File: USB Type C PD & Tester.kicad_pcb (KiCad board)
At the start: 2 copper layers, 115 x 50 mm, 61 parts, among them J1 USB_B_Micro, J3 USB_C_Receptacle_USB2.0_14P, J4 Screw_Terminal_01x02, Q1 BSD840N, Q2 BSD840N, Q3 BSD840N, Q4 BSD840N, SW1 SW_Push, U1 MIC5504-1.2YM5, U2 STM32F072CBTx, U3 INA237, U4 INA237, U5 AD8606ARM, U6 FUSB302B01MPX

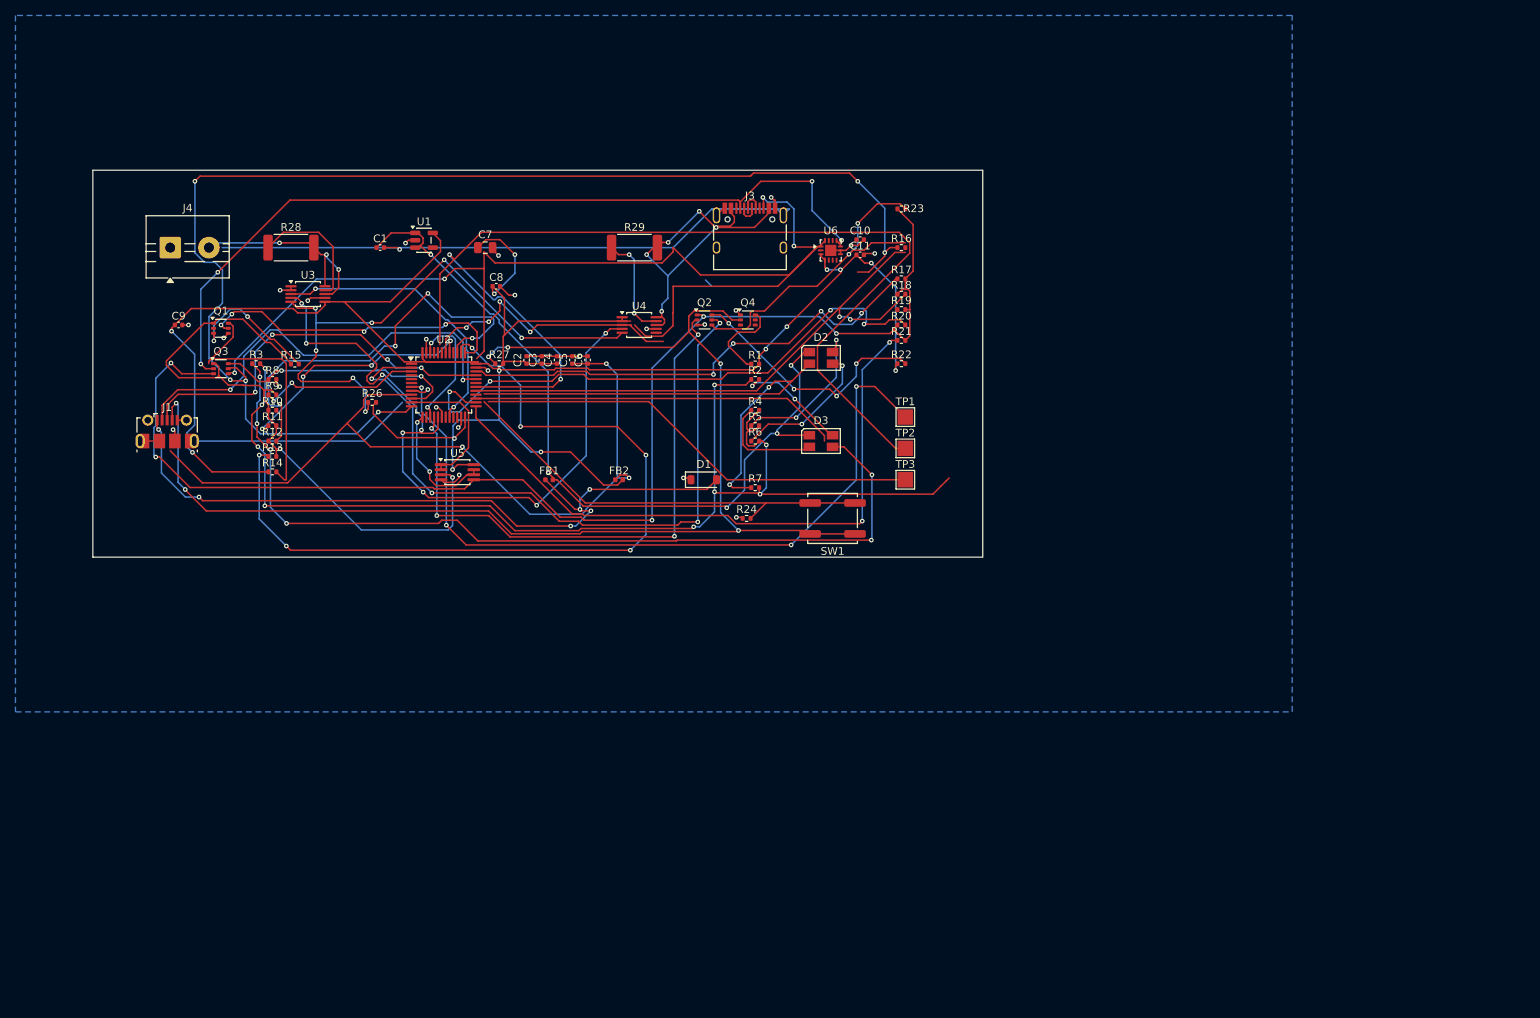
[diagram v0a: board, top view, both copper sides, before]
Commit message: Add files via upload
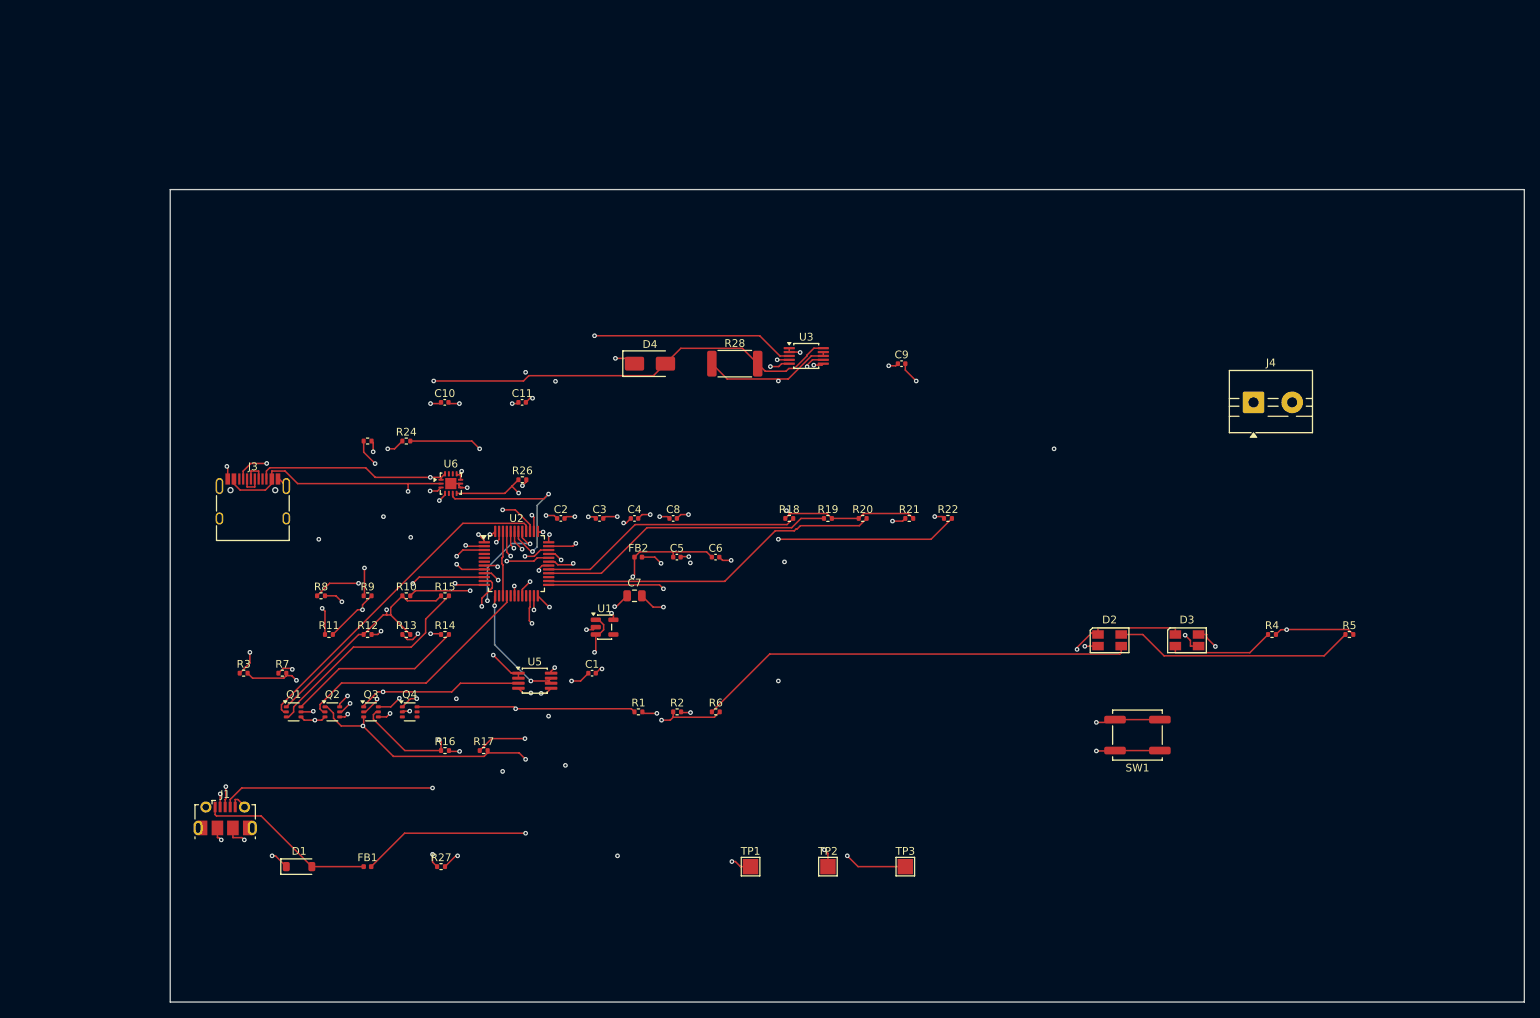
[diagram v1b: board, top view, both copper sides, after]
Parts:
- removed R29: 0.012Ω, Resistor_SMD:R_2512_6332Metric
- removed U4: INA237, Package_SO:VSSOP-10_3x3mm_P0.5mm
- added D4: D_TVS, Diode_SMD:D_SMA, F.Cu at (107.0, 65.0)
- moved J4 141.4 mm to (185.0, 70.0)
- moved C9 93.6 mm to (139.5, 65.0)
- moved R16 87.8 mm to (80.5, 115.0)
- moved R17 81.4 mm to (85.5, 115.0)
- moved R5 81.4 mm to (197.4, 100.0)
- moved R23 75.2 mm to (70.5, 75.0)
- moved J3 73.2 mm to (55.7, 84.0)
- moved R4 72.8 mm to (187.4, 100.0)
- moved D1 72.4 mm to (61.6, 130.0)
- moved Q2 69.9 mm to (66.0, 110.0)
- moved Q4 66.9 mm to (76.0, 110.0)
- moved R7 65.6 mm to (59.5, 105.0)
- moved R27 65.4 mm to (80.0, 130.0)
- moved U3 64.9 mm to (127.2, 64.0)
- moved TP1 61.4 mm to (120.0, 130.0)
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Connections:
- R26 pad 1: /INA_SDA -> INA_SDA
- R28 pad 1: Net-(U3-Vin-) -> /VBUS_PLUG
- R28 pad 2: /VBUS_PLUG -> /VBUS_RECEP
- U2 pad 17: /VCONN_ALERT_L -> unconnected-(U2-PA7-Pad17)
- U2 pad 42: /INA_SCL -> INA_SCL
- U2 pad 43: /INA_SDA -> INA_SDA
- U3 pad 10: /VBUS_PLUG -> /VBUS_RECEP
- U3 pad 4: /VCONN_ALERT_L -> INA_SDA
- U3 pad 5: /INA_SDA -> INA_SCL
- U3 pad 9: Net-(U3-Vin-) -> /VBUS_PLUG
- U6 pad 6: /INA_SCL -> INA_SCL
- U6 pad 7: /INA_SDA -> INA_SDA
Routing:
- net +3V3: track 287.6 -> 33.0 mm, vias 14 -> 23
- net /CC2_EN: track 167.9 -> 38.2 mm, vias 6 -> 2
- net GND: track 172.6 -> 70.9 mm, vias 25 -> 31
- net /VCONN_ALERT_L: track 91.3 -> 0.00 mm, vias 8 -> 0
- net /CC2_RECEP: track 149.3 -> 59.6 mm, vias 4 -> 2
- net /INA_SDA: track 74.8 -> 0.00 mm, vias 7 -> 0
- net Net-(R24-Pad2): track 56.2 -> 129.6 mm, vias 0 -> 3
- net /CC1_RPUSB: track 106.1 -> 34.5 mm, vias 6 -> 3
- net INA_SCL: track 0.00 -> 71.0 mm, vias 0 -> 4
- net INA_SDA: track 0.00 -> 70.9 mm, vias 0 -> 4
- net Net-(D1-A): track 93.8 -> 23.0 mm, vias 6 -> 0
- net Net-(U2-VDDA): track 103.0 -> 33.6 mm, vias 3 -> 2
- net /UART_TX: track 145.1 -> 75.7 mm, vias 2 -> 3
- net Net-(Q2A-D): track 32.6 -> 100.2 mm, vias 4 -> 3
- net Net-(D3-RK): track 14.6 -> 75.7 mm
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- added copper zone on In2.Cu, net +3V3
- added copper zone on In1.Cu, net GND
- removed copper zone on B.Cu, net GND
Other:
- board size 115 x 50 mm -> 175 x 105 mm
- copper layers 2 -> 4
- board text removed: "${REFERENCE}"

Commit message: Add files via upload
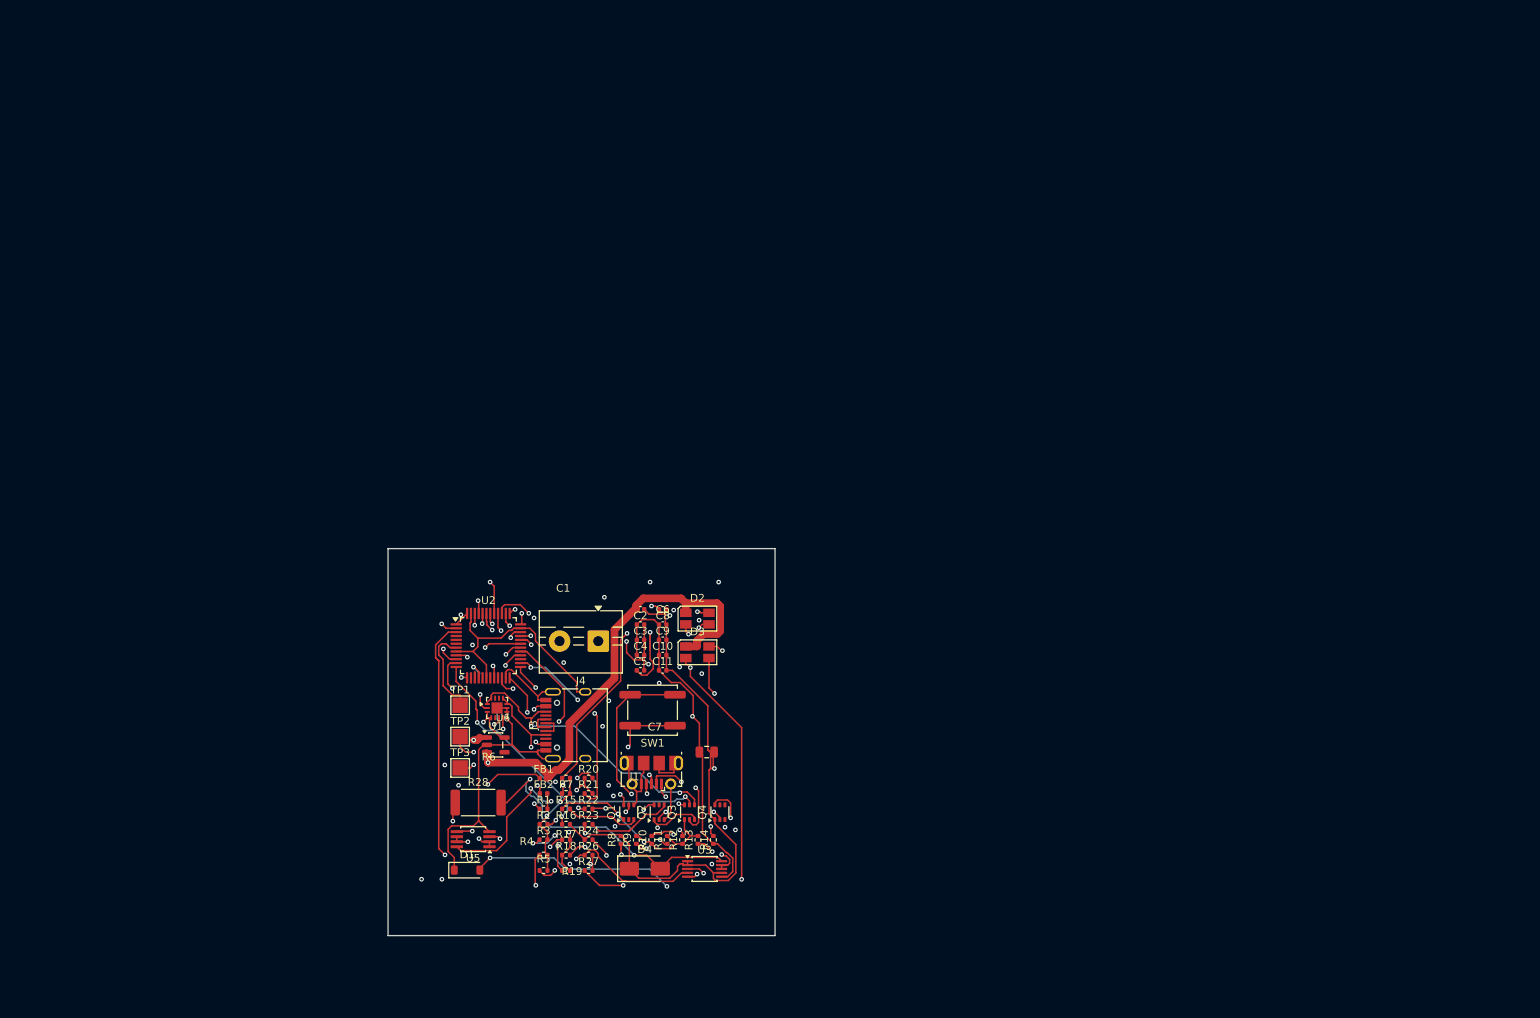
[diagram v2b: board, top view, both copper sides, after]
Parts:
- moved R5 108.5 mm to (93.2, 130.5)
- moved R4 98.4 mm to (93.2, 128.5)
- moved J4 90.1 mm to (100.3, 100.9), turned to 180 degrees
- moved U3 67.6 mm to (114.1, 130.3)
- moved R28 65.7 mm to (84.8, 121.7)
- moved D4 65.3 mm to (106.3, 130.3)
- moved D3 63.3 mm to (113.1, 102.3)
- moved SW1 62.7 mm to (107.3, 109.8)
- moved R22 59.7 mm to (99.1, 122.5)
- moved TP3 58.9 mm to (82.5, 117.2)
- moved R23 57.2 mm to (99.1, 124.5)
- moved R19 56.7 mm to (96.2, 130.5)
- moved R24 56.7 mm to (99.1, 126.5)
- moved J1 55.4 mm to (107.2, 117.9), turned to 180 degrees
- moved R21 54.6 mm to (99.1, 120.6)
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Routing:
- net GND: track 70.9 -> 246.0 mm, vias 31 -> 2
- net /400: track 178.4 -> 35.7 mm, vias 5 -> 3
- net +3V3: track 33.0 -> 156.4 mm, vias 23 -> 9
- net /CC2: track 153.9 -> 50.3 mm
- net USB_B_ID: track 146.3 -> 47.9 mm
- net Net-(R24-Pad2): track 129.6 -> 34.3 mm, vias 3 -> 2
- net Net-(Q2A-D): track 100.2 -> 8.49 mm, vias 3 -> 2
- net Net-(D3-GK): track 127.8 -> 49.2 mm, vias 2 -> 6
- net Net-(D2-BK): track 107.7 -> 36.2 mm, vias 2 -> 3
- net +5V: track 134.9 -> 65.3 mm, vias 4 -> 2
- net /CC1_RA: track 18.8 -> 78.2 mm, vias 2 -> 4
- net /NRST: track 70.7 -> 11.9 mm, vias 3 -> 0
- net /UART_RX: track 81.4 -> 23.3 mm, vias 3 -> 2
- net /UART_TX: track 75.7 -> 22.7 mm, vias 3 -> 2
- net Net-(D3-BK): track 13.8 -> 63.2 mm, vias 0 -> 3
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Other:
- board size 175 x 105 mm -> 50 x 50 mm
